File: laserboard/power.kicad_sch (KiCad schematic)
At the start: 0 parts

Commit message: Laserboard backup
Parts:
- added C17, C18: 10u, Capacitor_SMD:C_0805_2012Metric, symbol Device:C
- added J2: USB_B_Micro, RP2040_minimal:USB_Micro-B_Amphenol_10103594-0001LF_Horizontal_modified, symbol Connector:USB_B_Micro
- added U5: NCP1117-3.3_SOT223, Package_TO_SOT_SMD:SOT-223-3_TabPin2, symbol Regulator_Linear:NCP1117-3.3_SOT223
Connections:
- new net +3V3: C18.1, U5.2 (VO)
- new net GND: C17.2, C18.2, J2.5 (GND), J2.6 (Shield), U5.1 (GND)
- new net MCU_USB_D+: J2.3 (D+)
- new net MCU_USB_D-: J2.2 (D-)
- new net VBUS: C17.1, J2.1 (VBUS), U5.3 (VI)
- no-connect marks 0 -> 1
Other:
- note added: "Power"

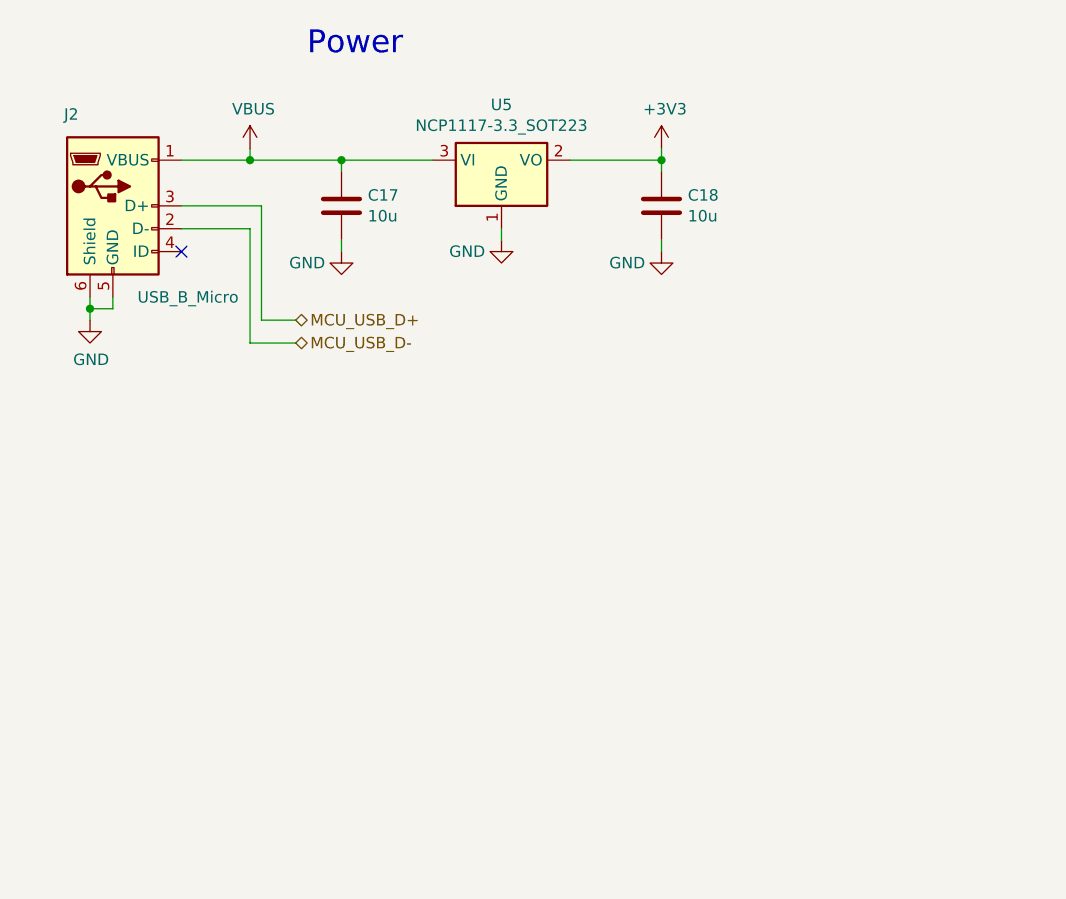
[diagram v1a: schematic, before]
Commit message: Update
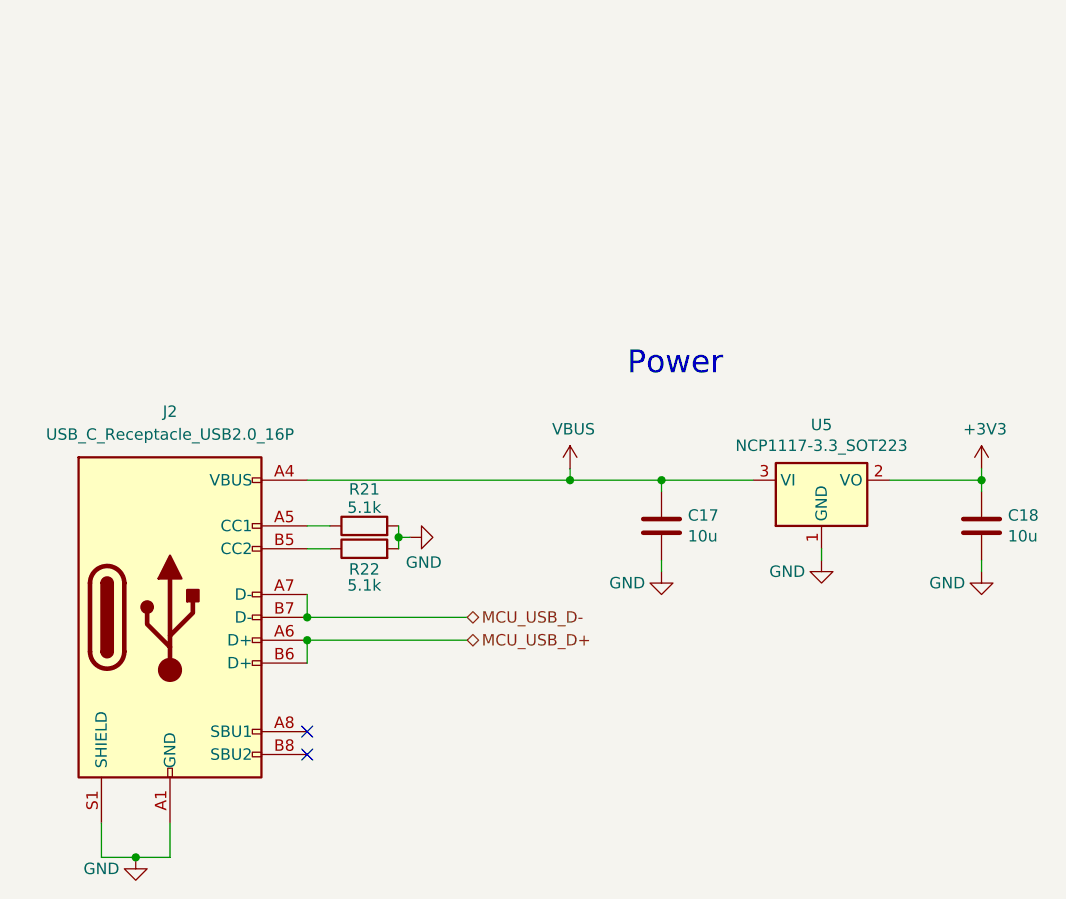
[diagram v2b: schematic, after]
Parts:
- removed J2: USB_B_Micro, RP2040_minimal:USB_Micro-B_Amphenol_10103594-0001LF_Horizontal_modified, symbol Connector:USB_B_Micro
- added J2: USB_C_Receptacle_USB2.0_16P, Connector_USB:USB_C_Receptacle_GCT_USB4105-xx-A_16P_TopMnt_Horizontal, symbol Connector:USB_C_Receptacle_USB2.0_16P
- added R21, R22: 5.1k, symbol Device:R
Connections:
- net GND: now also J2.A1 (GND), J2.A12 (GND), J2.B1 (GND), J2.B12 (GND), J2.S1 (SHIELD), R21.2, R22.2
- net MCU_USB_D+: now also J2.A6 (D+), J2.B6 (D+)
- net MCU_USB_D-: now also J2.A7 (D-), J2.B7 (D-)
- net VBUS: now also J2.A4 (VBUS), J2.A9 (VBUS), J2.B4 (VBUS), J2.B9 (VBUS)
- new net: J2.A5 (CC1), R21.1
- new net: J2.B5 (CC2), R22.1
- no-connect marks 1 -> 2
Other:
- moved on the sheet: C17, C18, U5
